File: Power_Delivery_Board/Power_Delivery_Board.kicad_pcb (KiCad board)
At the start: 2 copper layers, 53 x 45 mm, 49 parts, among them IC1 STUSB4500QTR, J1 USB C, J2 IO pins, J3 Power Output, J4 IO Pins, J5 Qwiic, Q1 STL6P3LLH6

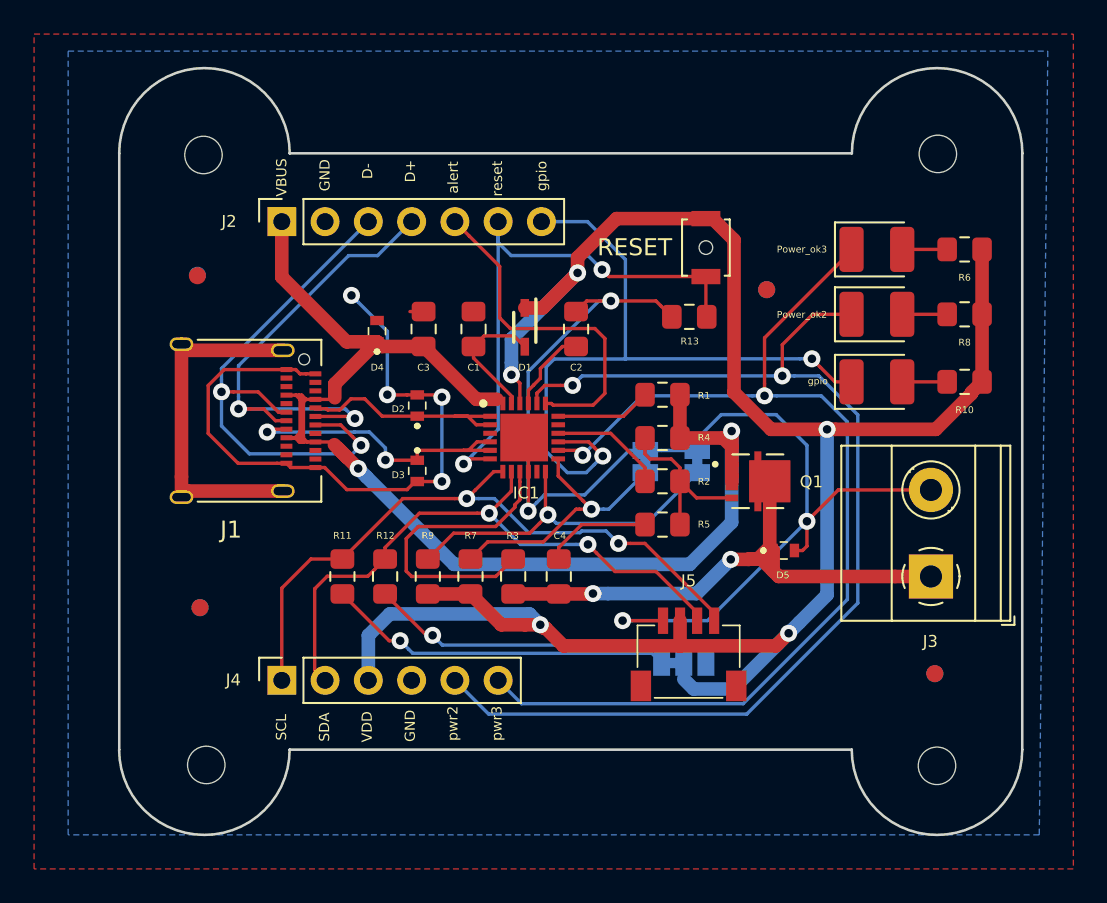
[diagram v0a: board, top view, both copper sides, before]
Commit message: Arreglo borde PCB
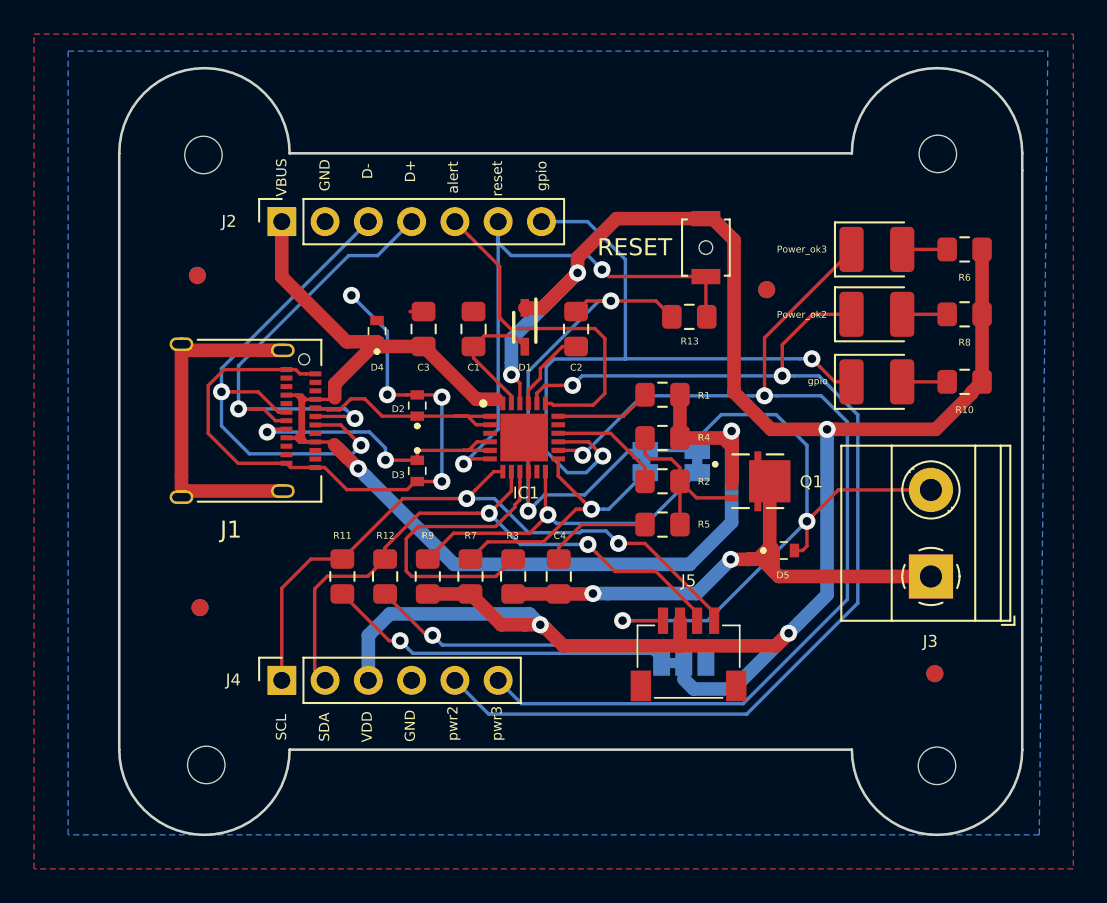
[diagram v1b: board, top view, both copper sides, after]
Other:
- outline, holes or cut-outs redrawn
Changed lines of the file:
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@@
   (general
     (thickness 1.6)
-    (drawings 38)
+    (drawings 39)
     (tracks 496)
     (zones 0)
@@
     (44 Edge.Cuts user)
     (45 Margin user)
-    (46 B.CrtYd user hide)
-    (47 F.CrtYd user hide)
+    (46 B.CrtYd user)
+    (47 F.CrtYd user)
     (48 B.Fab user hide)
     (49 F.Fab user hide)
@@
       (xy -3.2512 3.335866) (xy 3.2512 3.335866) (xy 3.2512 -3.3528)) (layer B.SilkS) (width 0.01))
   )
-  (gr_arc (start 125 60) (end 130.004057 60) (angle -180) (layer Edge.Cuts) (width 0.15))
+  (gr_line (start 130 95) (end 163 95) (layer Edge.Cuts) (width 0.15))
+  (gr_line (start 130 60) (end 163 60) (layer Edge.Cuts) (width 0.15))
+  (gr_arc (start 168 95) (end 163 95) (angle -180) (layer Edge.Cuts) (width 0.15))
+  (gr_arc (start 125 95) (end 120 95) (angle -180) (layer Edge.Cuts) (width 0.15))
+  (gr_arc (start 125 60) (end 130 60) (angle -180) (layer Edge.Cuts) (width 0.15))
+  (gr_arc (start 168 60) (end 173 60) (angle -180) (layer Edge.Cuts) (width 0.15))
+  (gr_line (start 120 95) (end 120 60) (layer Edge.Cuts) (width 0.15))
+  (gr_line (start 173 61) (end 173 60) (layer Edge.Cuts) (width 0.15))
+  (gr_line (start 173 95) (end 173 61) (layer Edge.Cuts) (width 0.15))
   (gr_text "Errores DRC aprobados:\n- Pad near pad:\n    @(129.602mm, 79.822mm) Pad S1 on F.Cu Internal, Non-copper of J1\n    @(130.852mm, 79.292mm) Pad on F.Cu, B.Cu Internal, Non-copper of J1\n- Pad near pad:\n    @(150.876mm, 77.440mm) Pad 2 on B.Cu Non-copper of J1\n    @(150.876mm, 78.740mm) Pad 1 on B.Cu, Non-copper of J1\n- Pad near pad:\n    @(151.832mm, 89.916mm) Pad 1 on B.Cu Non-copper of J1\n    @(153.132mm, 89.916mm) Pad 2 on B.Cu, Non-copper of J1\n- Pad near pad:\n    @(153.924mm, 77.440mm) Pad 2 on B.Cu Non-copper of J1\n    @(153.924mm, 78.740mm) Pad 1 on B.Cu, Non-copper of J1" (at 117 124) (layer Cmts.User)
     (effects (font (size 1.5 1.5) (thickness 0.3)) (justify left))
@@
     (effects (font (size 0.6 0.6) (thickness 0.15)))
   )
-  (gr_line (start 163 60) (end 130 60) (layer Edge.Cuts) (width 0.15))
-  (gr_arc (start 168.004057 60) (end 173.008114 60) (angle -180) (layer Edge.Cuts) (width 0.15))
-  (gr_line (start 130 95) (end 163 95) (layer Edge.Cuts) (width 0.15))
-  (gr_arc (start 124.995943 95) (end 119.991886 95) (angle -180) (layer Edge.Cuts) (width 0.15))
-  (gr_arc (start 167.995943 95) (end 162.991886 95) (angle -180) (layer Edge.Cuts) (width 0.15))
-  (gr_line (start 173 60) (end 173 95) (layer Edge.Cuts) (width 0.15))
-  (gr_line (start 120 60) (end 120 95) (layer Edge.Cuts) (width 0.15))
   (gr_text "Se utilizaron las capacidades del fabricante Ernesto Mayer \n(documentación en la raíz del proyecto)" (at 193 55) (layer Cmts.User)
     (effects (font (size 1.5 1.5) (thickness 0.3)) (justify left))
@@
     (effects (font (size 1.5 1.5) (thickness 0.3)) (justify left))
   )
-  (dimension 34 (width 0.3) (layer Dwgs.User)
-    (gr_text "34.000 mm" (at 180.1 78 90) (layer Dwgs.User)
+  (dimension 35 (width 0.3) (layer Dwgs.User)
+    (gr_text "35.000 mm" (at 180.1 77.5 90) (layer Dwgs.User)
       (effects (font (size 1.5 1.5) (thickness 0.3)))
     )
-    (feature1 (pts (xy 173 61) (xy 178.586421 61)))
+    (feature1 (pts (xy 173 60) (xy 178.586421 60)))
     (feature2 (pts (xy 173 95) (xy 178.586421 95)))
-    (crossbar (pts (xy 178 95) (xy 178 61)))
-    (arrow1a (pts (xy 178 61) (xy 178.586421 62.126504)))
-    (arrow1b (pts (xy 178 61) (xy 177.413579 62.126504)))
+    (crossbar (pts (xy 178 95) (xy 178 60)))
+    (arrow1a (pts (xy 178 60) (xy 178.586421 61.126504)))
+    (arrow1b (pts (xy 178 60) (xy 177.413579 61.126504)))
     (arrow2a (pts (xy 178 95) (xy 178.586421 93.873496)))
     (arrow2b (pts (xy 178 95) (xy 177.413579 93.873496)))
